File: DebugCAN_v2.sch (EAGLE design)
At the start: 58 parts, among them J1 8P8C-LED, J2 XT60PW-M, J3 MA04-1, J4 10118192-0001LF, J5 8P8C-LED, J6 8P8C-LED, J7 8P8C-LED, U1 STM32F302C, U2 NCV7351D1E, U3 SI8621AB-B-IS, U4 AP2127N-3.3TRG1, U5 78L05F, U6 TLP291, X1 CSTCE8M00G55

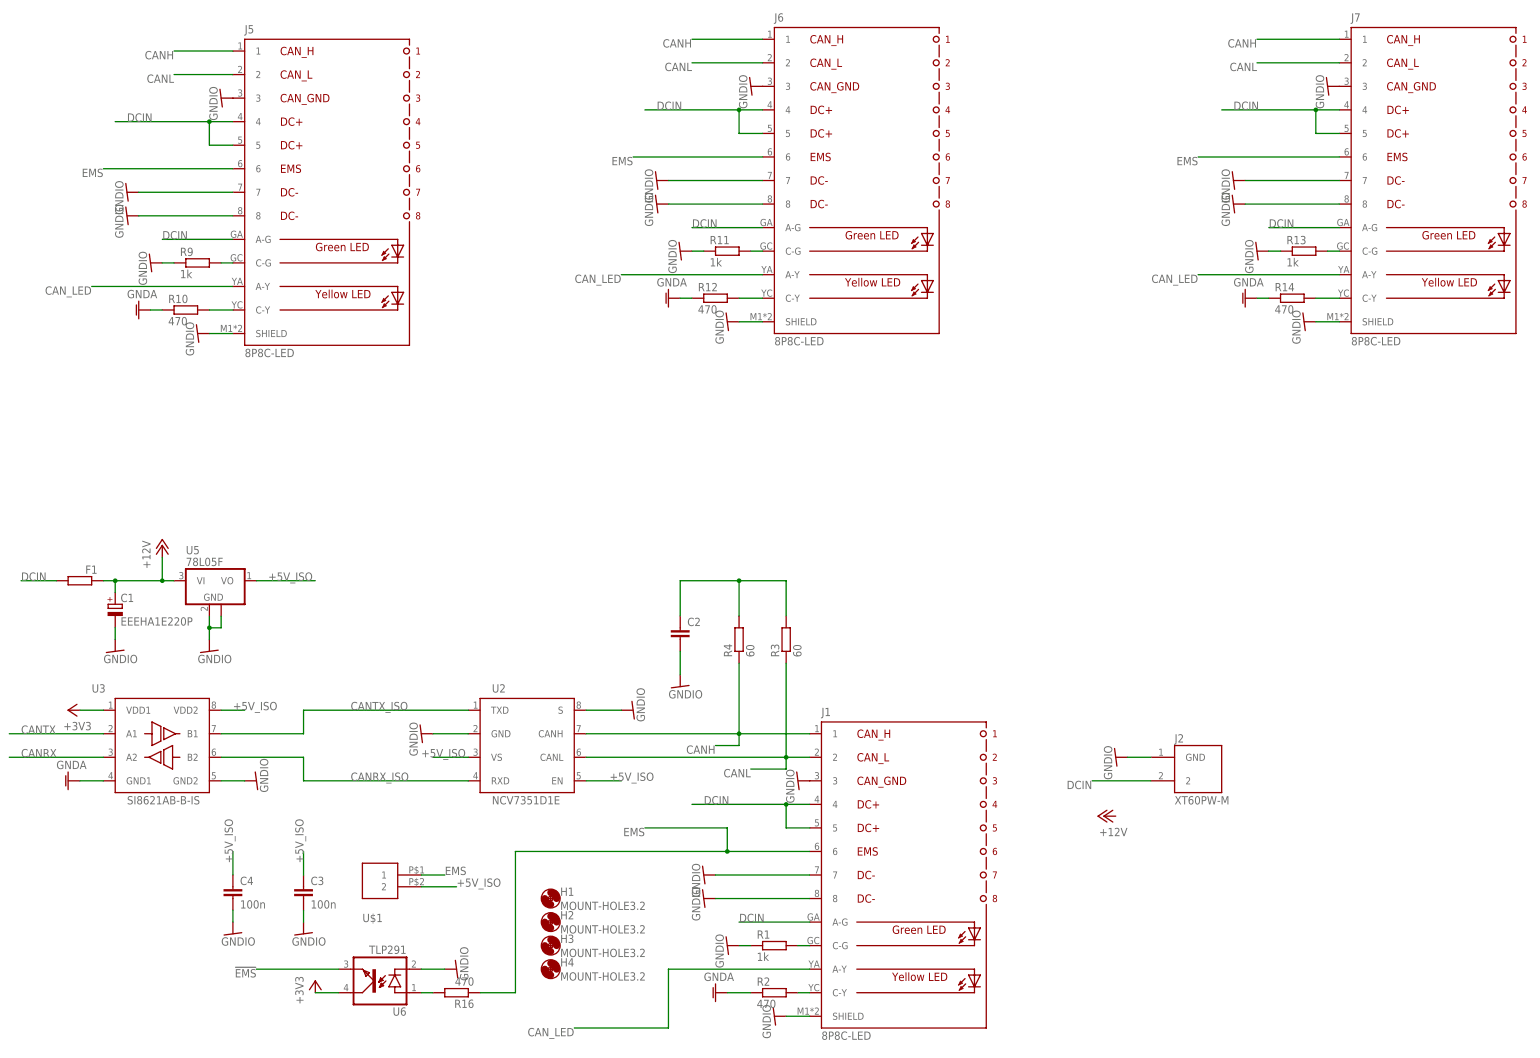
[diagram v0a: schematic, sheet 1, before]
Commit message: ver.2 update
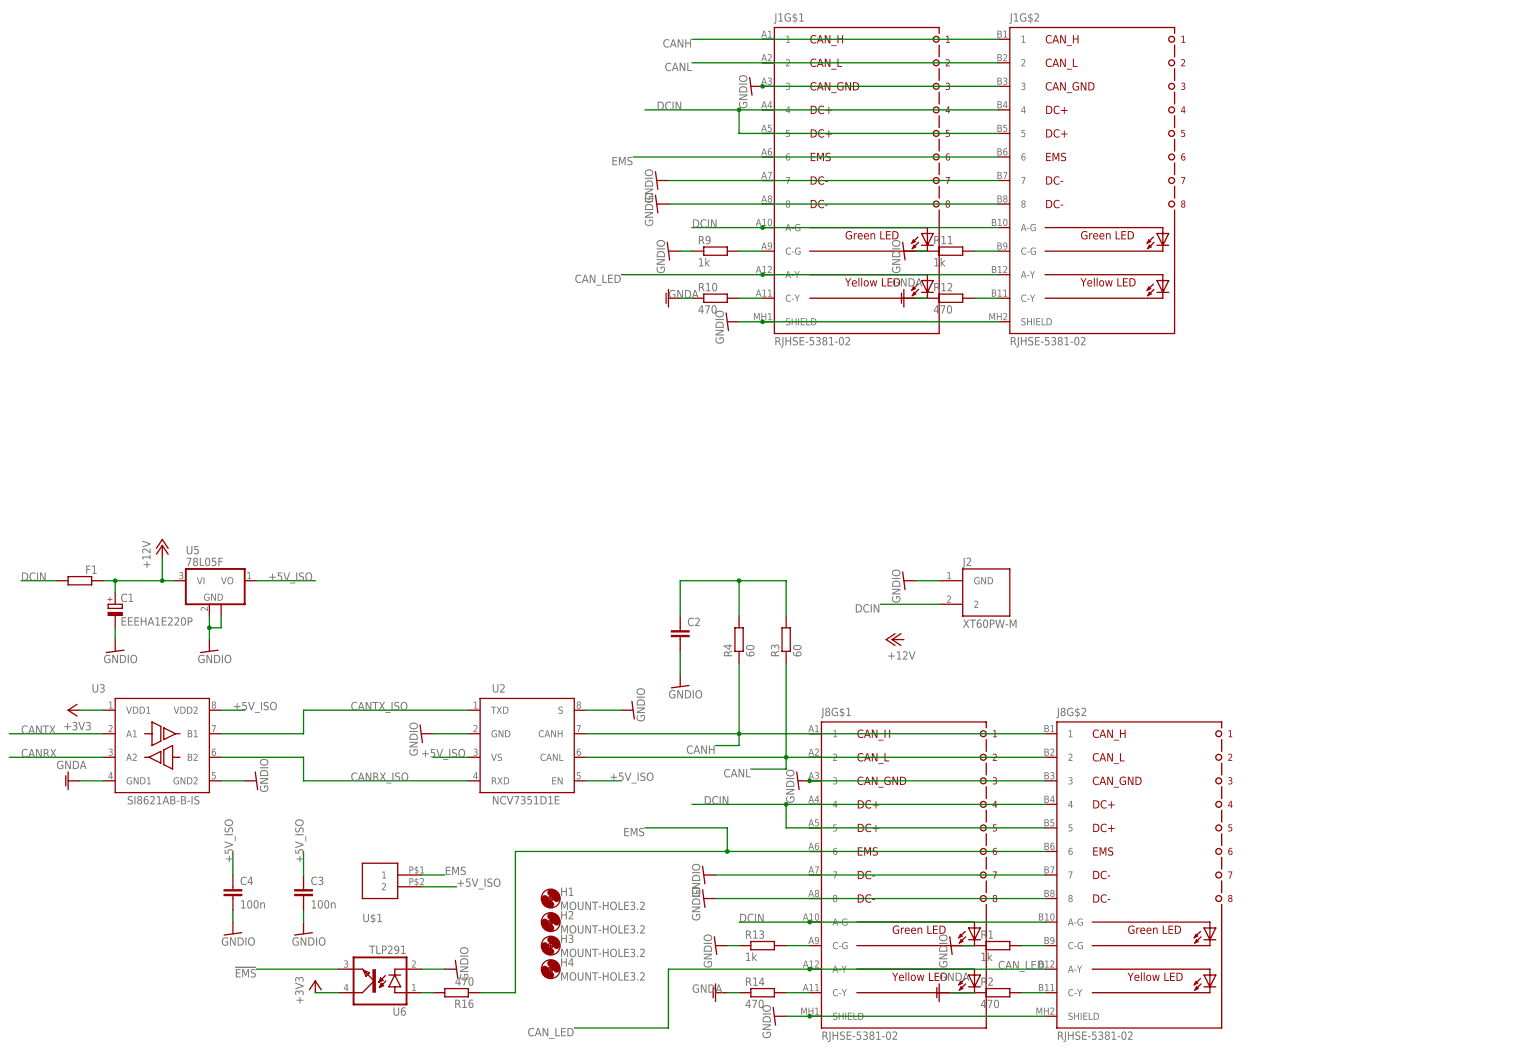
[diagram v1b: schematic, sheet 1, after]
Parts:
- removed J5, J6, J7: 8P8C-LED, con-rj45:8P8C-LED
- added J8: RJHSE-5381-02, con-rj45:RJHSE-5381-02
- J1: value 8P8C-LED -> RJHSE-5381-02; device con-rj45:8P8C-LED -> con-rj45:RJHSE-5381-02
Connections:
- removed net N$15: J7.C-Y, R14.2
- new net N$1: J1G$1.C-G, R9.2
- net CANH: now also J1G$1.1, J1G$2.1, J8G$1.1, J8G$2.1; no longer J1.1, J5.1, J6.1, J7.1
- net CANL: now also J1G$1.2, J1G$2.2, J8G$1.2, J8G$2.2; no longer J1.2, J5.2, J6.2, J7.2
- net CAN_LED: now also J1G$1.A-Y, J1G$2.A-Y, J8G$1.A-Y, J8G$2.A-Y; no longer J1.A-Y, J5.A-Y, J6.A-Y, J7.A-Y
- net DCIN: now also J1G$1.4, J1G$1.5, J1G$1.A-G, J1G$2.4, J1G$2.5, J1G$2.A-G, J8G$1.4, J8G$1.5, J8G$1.A-G, J8G$2.4, J8G$2.5, J8G$2.A-G; no longer J1.4, J1.5, J1.A-G, J5.4, J5.5, J5.A-G, J6.4, J6.5, J6.A-G, J7.4, J7.5, J7.A-G
- net EMS: now also J1G$1.6, J1G$2.6, J8G$1.6, J8G$2.6; no longer J1.6, J5.6, J6.6, J7.6
- net GNDIO: now also J1G$1.3, J1G$1.7, J1G$1.8, J1G$1.SHIELD, J1G$2.3, J1G$2.7, J1G$2.8, J1G$2.SHIELD, J8G$1.3, J8G$1.7, J8G$1.8, J8G$1.SHIELD, J8G$2.3, J8G$2.7, J8G$2.8, J8G$2.SHIELD; no longer J1.3, J1.7, J1.8, J1.SHIELD, J5.3, J5.7, J5.8, J5.SHIELD, J6.3, J6.7, J6.8, J6.SHIELD, J7.3, J7.7, J7.8, J7.SHIELD
- net N$10: now also J1G$2.C-Y, R12.2; no longer J5.C-Y, R10.2
- net N$12: now also J1G$2.C-G; no longer J6.C-G
- net N$13: now also J8G$1.C-Y, R14.2; no longer J6.C-Y, R12.2
- net N$14: now also J8G$1.C-G; no longer J7.C-G
- net N$3: now also J8G$2.C-G; no longer J1.C-G
- net N$4: now also J8G$2.C-Y; no longer J1.C-Y
- net N$9: now also J1G$1.C-Y, R10.2; no longer J5.C-G, R9.2
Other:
- moved on the sheet: J1G$1, J2, R1, R10, R11, R12, R13, R14, R2, R9
